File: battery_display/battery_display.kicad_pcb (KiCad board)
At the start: 2 copper layers, 100 x 60 mm, 30 parts, among them J1 FH34SRJ-24S-0.5SH_99_, J2 Screw_Terminal_2x2.54, Q1 ZXM61N03F, Q2 ZXM61N03F, SW1 Button-THT - 2-1825910-7, U1 LDO40LPU33RY

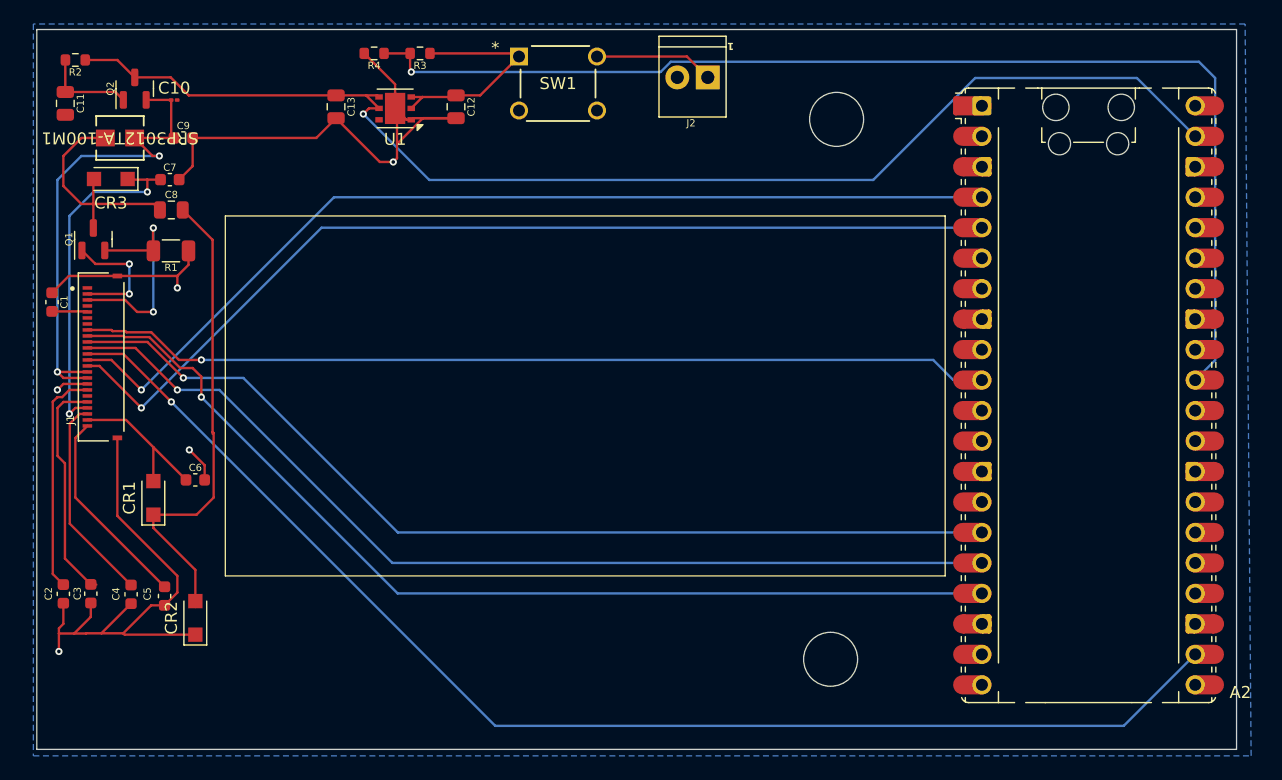
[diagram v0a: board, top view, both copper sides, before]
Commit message: Reapply "Added some small fixes"
This reverts commit d414565db0f35087673e5f9750bdaf74336bf2be.
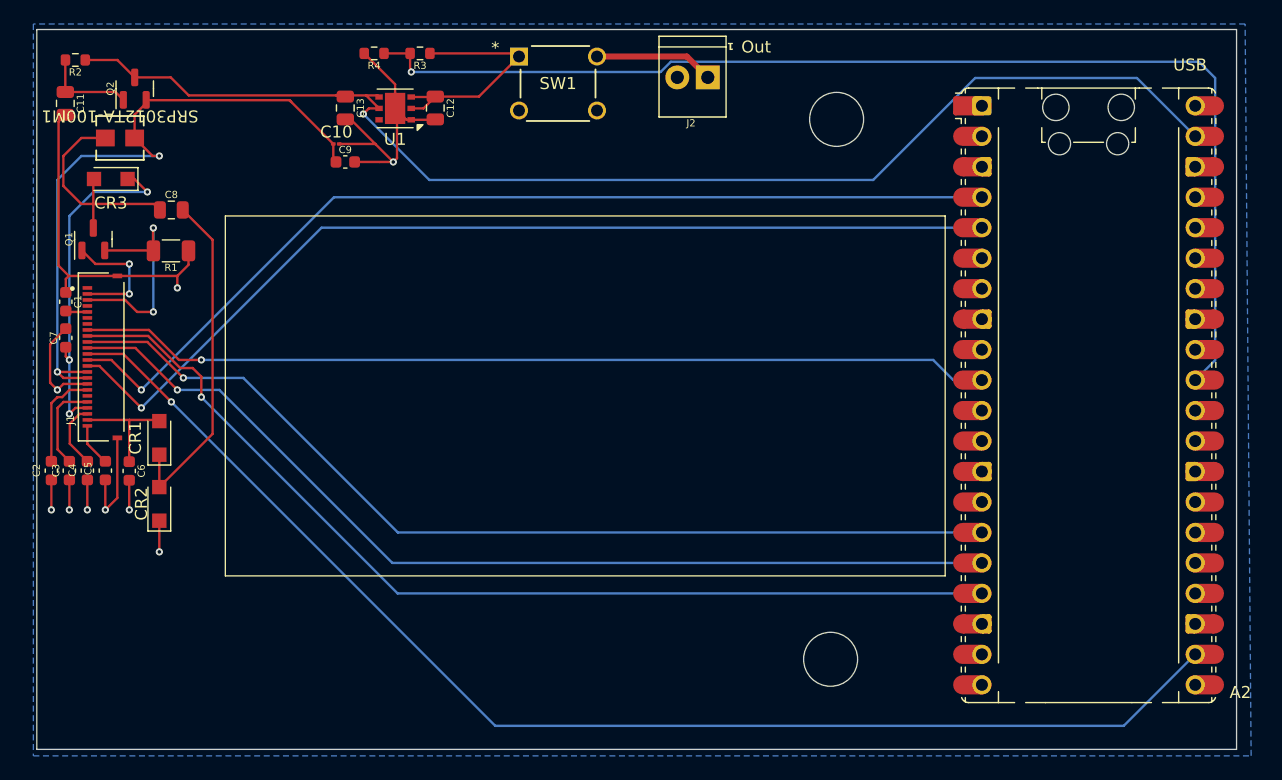
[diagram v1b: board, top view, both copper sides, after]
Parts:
- moved C7 15.8 mm to (157.7, 55.7), turned to 90 degrees
- moved C10 14.0 mm to (180.2, 39.5)
- moved C9 13.6 mm to (181.0, 41.0)
- moved C5 11.6 mm to (161.0, 66.7)
- moved C4 10.9 mm to (159.5, 66.7)
- moved C3 10.4 mm to (158.0, 66.7)
- moved C2 10.3 mm to (156.5, 66.7)
- moved CR2 9.96 mm to (165.5, 69.5)
- moved C6 5.56 mm to (163.0, 66.8), turned to -90 degrees
- moved CR1 5.02 mm to (165.5, 64.0)
- moved C12 1.73 mm to (188.5, 36.5)
- moved C1 1.15 mm to (157.7, 52.6)
- moved C13 0.78 mm to (181.0, 36.5)
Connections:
- net /vcc renamed /12-16V
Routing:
- net GND: track 107.9 -> 84.1 mm, vias 5 -> 9
- net /Display VDDD: track 41.9 -> 55.7 mm
- net Net-(C5-Pad2): track 16.9 -> 3.60 mm
- net Net-(C4-Pad2): track 17.4 -> 5.55 mm
- net Net-(C3-Pad2): track 18.9 -> 7.55 mm
- net Net-(C8-Pad2): track 40.0 -> 28.7 mm
- net Net-(C2-Pad2): track 18.9 -> 8.31 mm
- net Net-(C6-Pad1): track 13.1 -> 9.52 mm
- net Net-(C1-Pad2): track 2.96 -> 1.89 mm
- net /voltage divider: track 19.3 -> 20.3 mm
- net Net-(C7-Pad1): track 29.4 -> 28.9 mm, vias 2 -> 3
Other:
- board text added: "Out"
- board text added: "USB"

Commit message: Revert "Added some small fixes"
This reverts commit 59b639d84f345d5fabc6edbb6fa9331222a6e139.
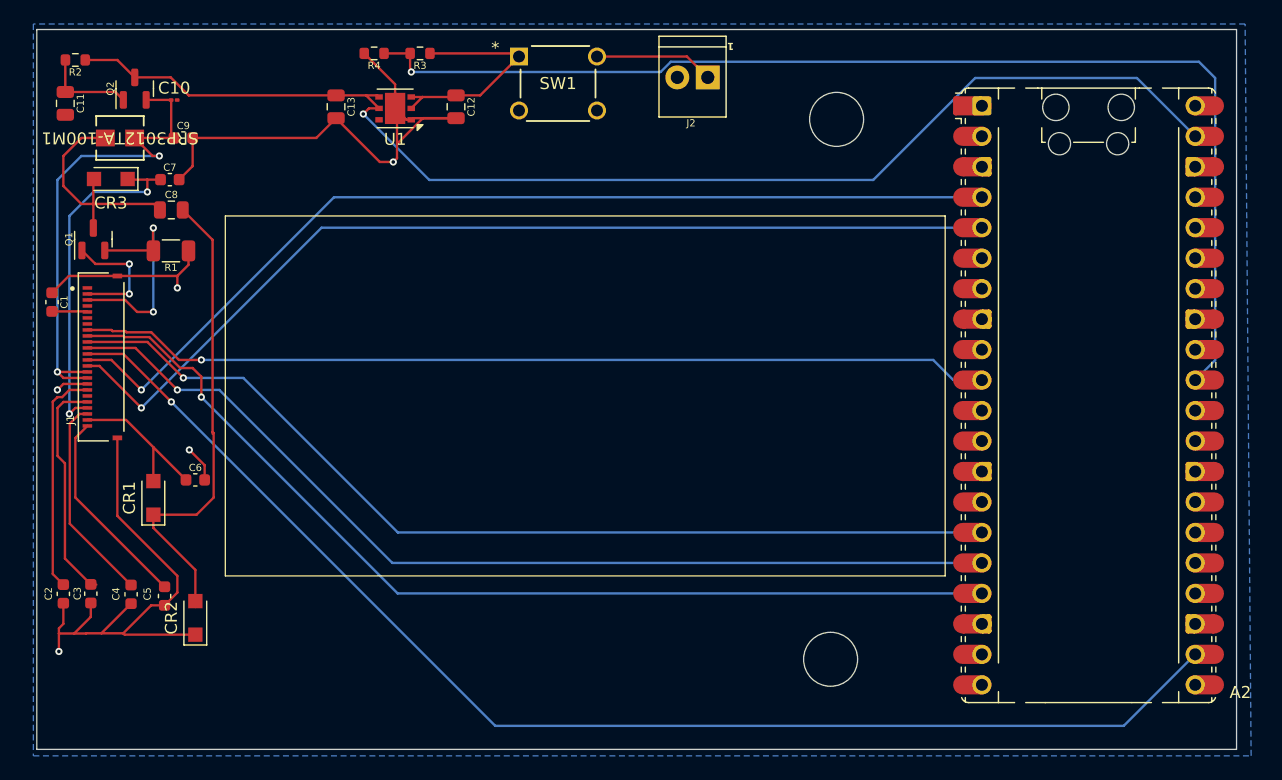
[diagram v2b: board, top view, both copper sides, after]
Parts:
- moved C7 15.8 mm to (166.4, 42.5), turned to 0 degrees
- moved C10 14.0 mm to (166.7, 35.8)
- moved C9 13.6 mm to (167.5, 39.0)
- moved C5 11.6 mm to (165.9, 77.2)
- moved C4 10.9 mm to (163.1, 77.0)
- moved C3 10.4 mm to (159.8, 77.0)
- moved C2 10.3 mm to (157.5, 77.0)
- moved CR2 9.96 mm to (168.5, 79.0)
- moved C6 5.56 mm to (168.5, 67.5), turned to 0 degrees
- moved CR1 5.02 mm to (165.0, 69.0)
- moved C12 1.73 mm to (190.2, 36.4)
- moved C1 1.15 mm to (156.6, 52.7)
- moved C13 0.78 mm to (180.2, 36.4)
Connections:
- net /12-16V renamed /vcc
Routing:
- net GND: track 84.1 -> 107.9 mm, vias 9 -> 5
- net /Display VDDD: track 55.7 -> 41.9 mm
- net Net-(C5-Pad2): track 3.60 -> 16.9 mm
- net Net-(C4-Pad2): track 5.55 -> 17.4 mm
- net Net-(C3-Pad2): track 7.55 -> 18.9 mm
- net Net-(C8-Pad2): track 28.7 -> 40.0 mm
- net Net-(C2-Pad2): track 8.31 -> 18.9 mm
- net Net-(C6-Pad1): track 9.52 -> 13.1 mm
- net Net-(C1-Pad2): track 1.89 -> 2.96 mm
- net /voltage divider: track 20.3 -> 19.3 mm
- net Net-(C7-Pad1): track 28.9 -> 29.4 mm, vias 3 -> 2
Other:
- board text removed: "Out"
- board text removed: "USB"
